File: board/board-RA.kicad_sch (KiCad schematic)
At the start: 29 parts, among them J1 port attiny, J10 BMS Bat +, J11 BMS Bat gnd, J12 BMS out -, J13 BMS in +5v, J14 BMS in gnd, J15_C189893 BMS led charge ok, J16 Mp3 D1 led marche ok, J17_C189893 Haut parleur, J18_C189893 Batterie + et -, J19_C189893 BMS in + et -, J2 alim attiny, J20 BMS led charge ok, J21_C189893 Vers bouton vol - et next, J22_C189893 Mp3 D1 led marche ok, J23 on - off, J23-C189893 alim +5 gnd, J24 port 3-C265421, J3 alim mp3, J4 hp mp3, J5_C189893 vol - et next +, J6 step up out, J7 step up in +, J8 step up in -, J9 BMS out +

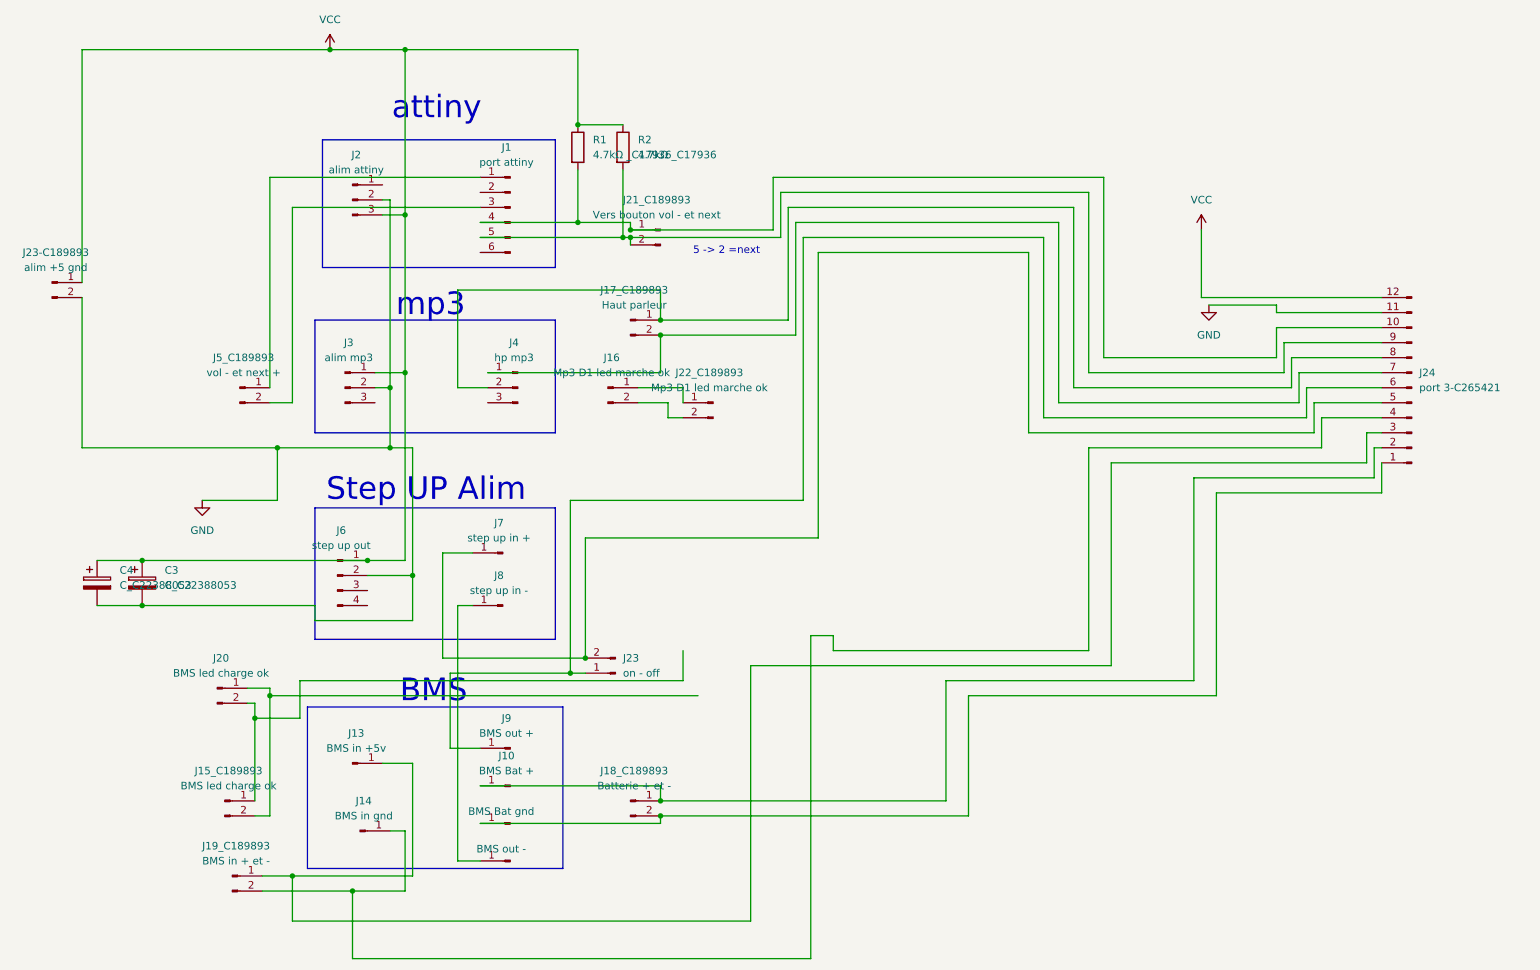
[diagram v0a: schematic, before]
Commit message: mise a jour pcb
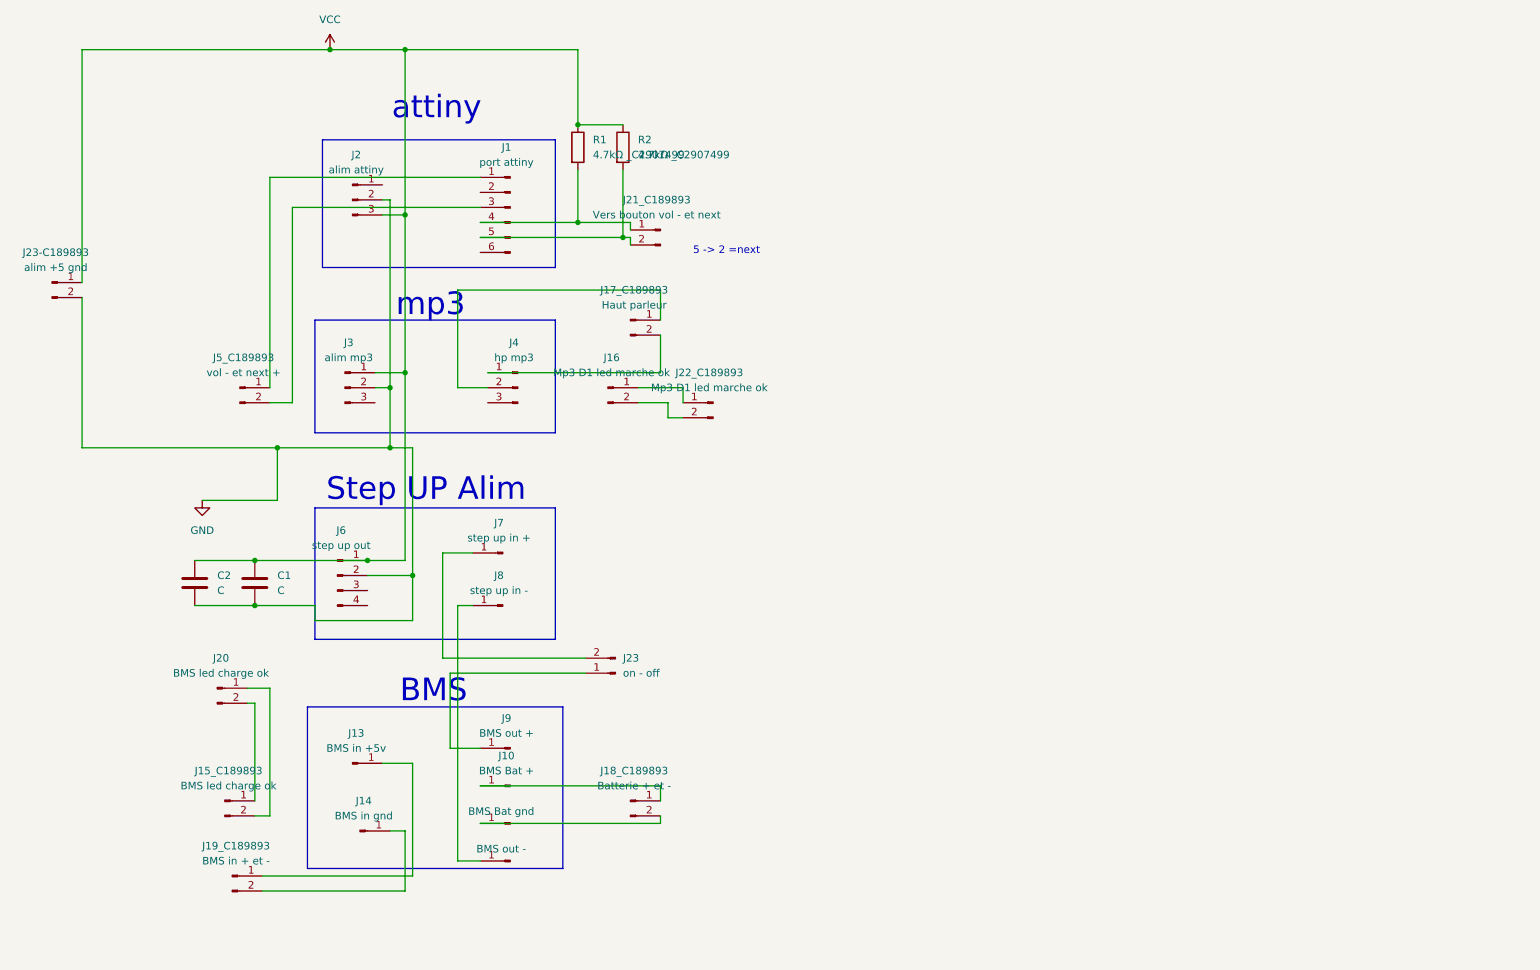
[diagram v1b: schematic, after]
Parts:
- removed C3, C4: C_C22388053, Capacitor_SMD:CP_Elec_6.3x7.7, symbol Device:C_Polarized
- removed J24: port 3-C265421, Connector_JST:JST_GH_SM12B-GHS-TB_1x12-1MP_P1.25mm_Horizontal, symbol Connector:Conn_01x12_Pin
- added C1, C2: C, Capacitor_THT:CP_Radial_D5.0mm_P2.50mm, symbol Device:C
- R1, R2: value 4.7kΩ _C17936 -> 4.7kΩ _C2907499
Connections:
- net GND: now also C1.2, C2.2
- net VCC: now also C1.1, C2.1
